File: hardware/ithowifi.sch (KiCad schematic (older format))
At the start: 20 parts, among them J1 Conn_02x03_Odd_Even, J2 conn, Q1 BSS138, Q2 BSS138, U1 WeMos_mini

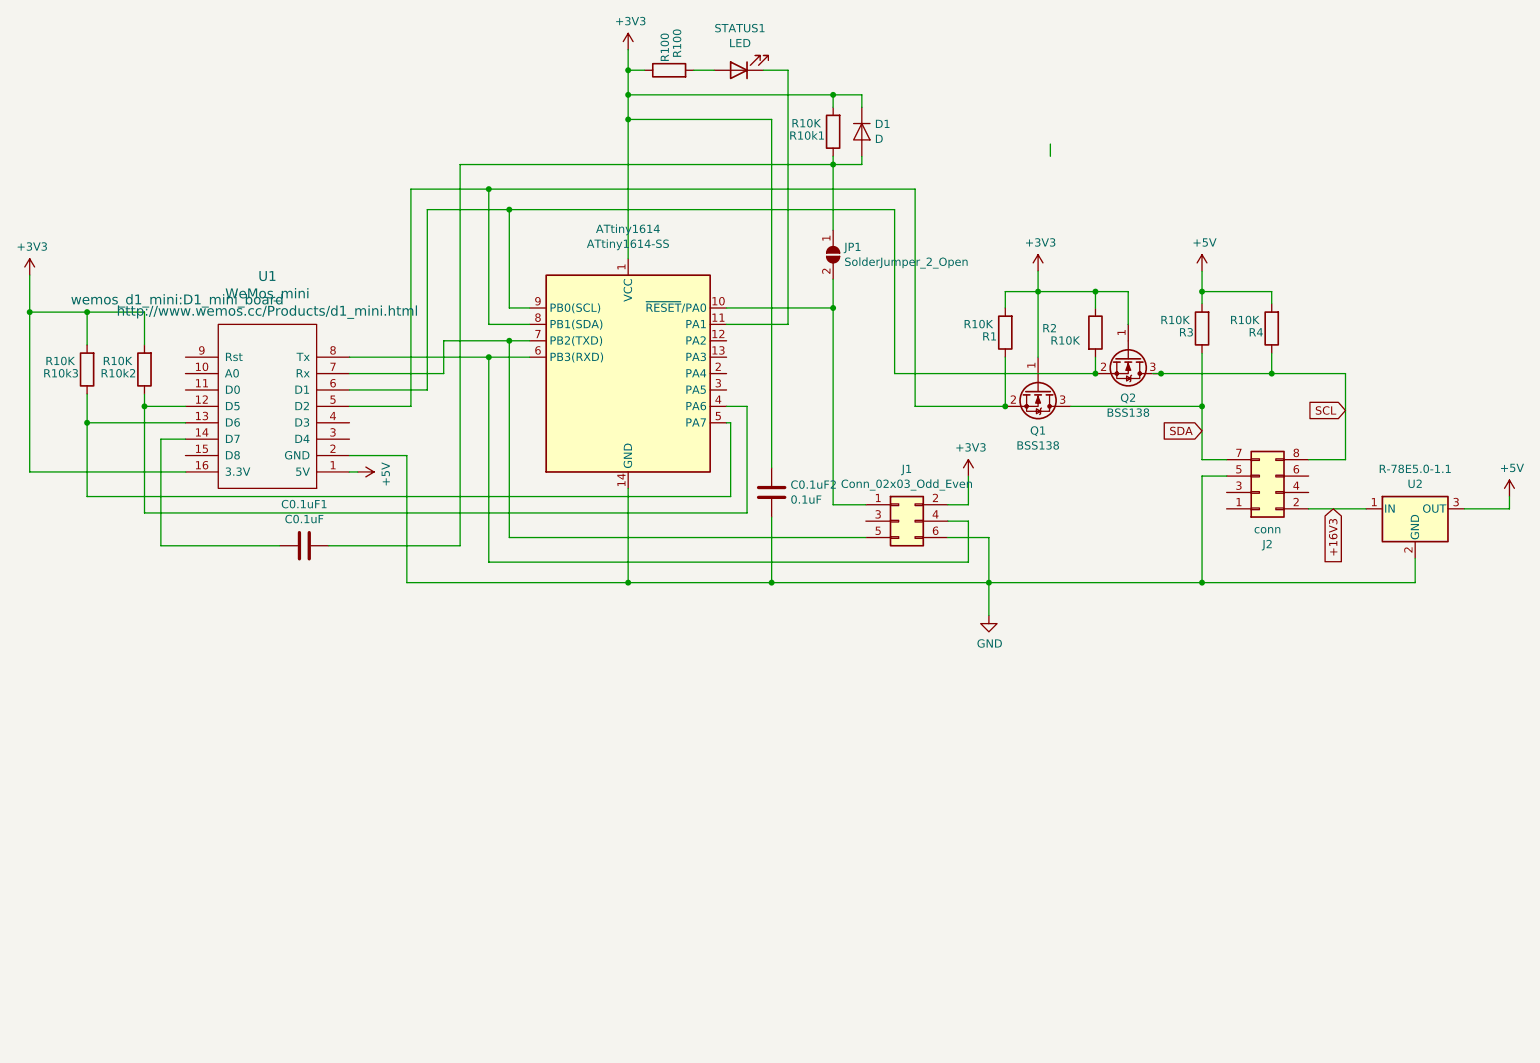
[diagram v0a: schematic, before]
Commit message: Test v2.0
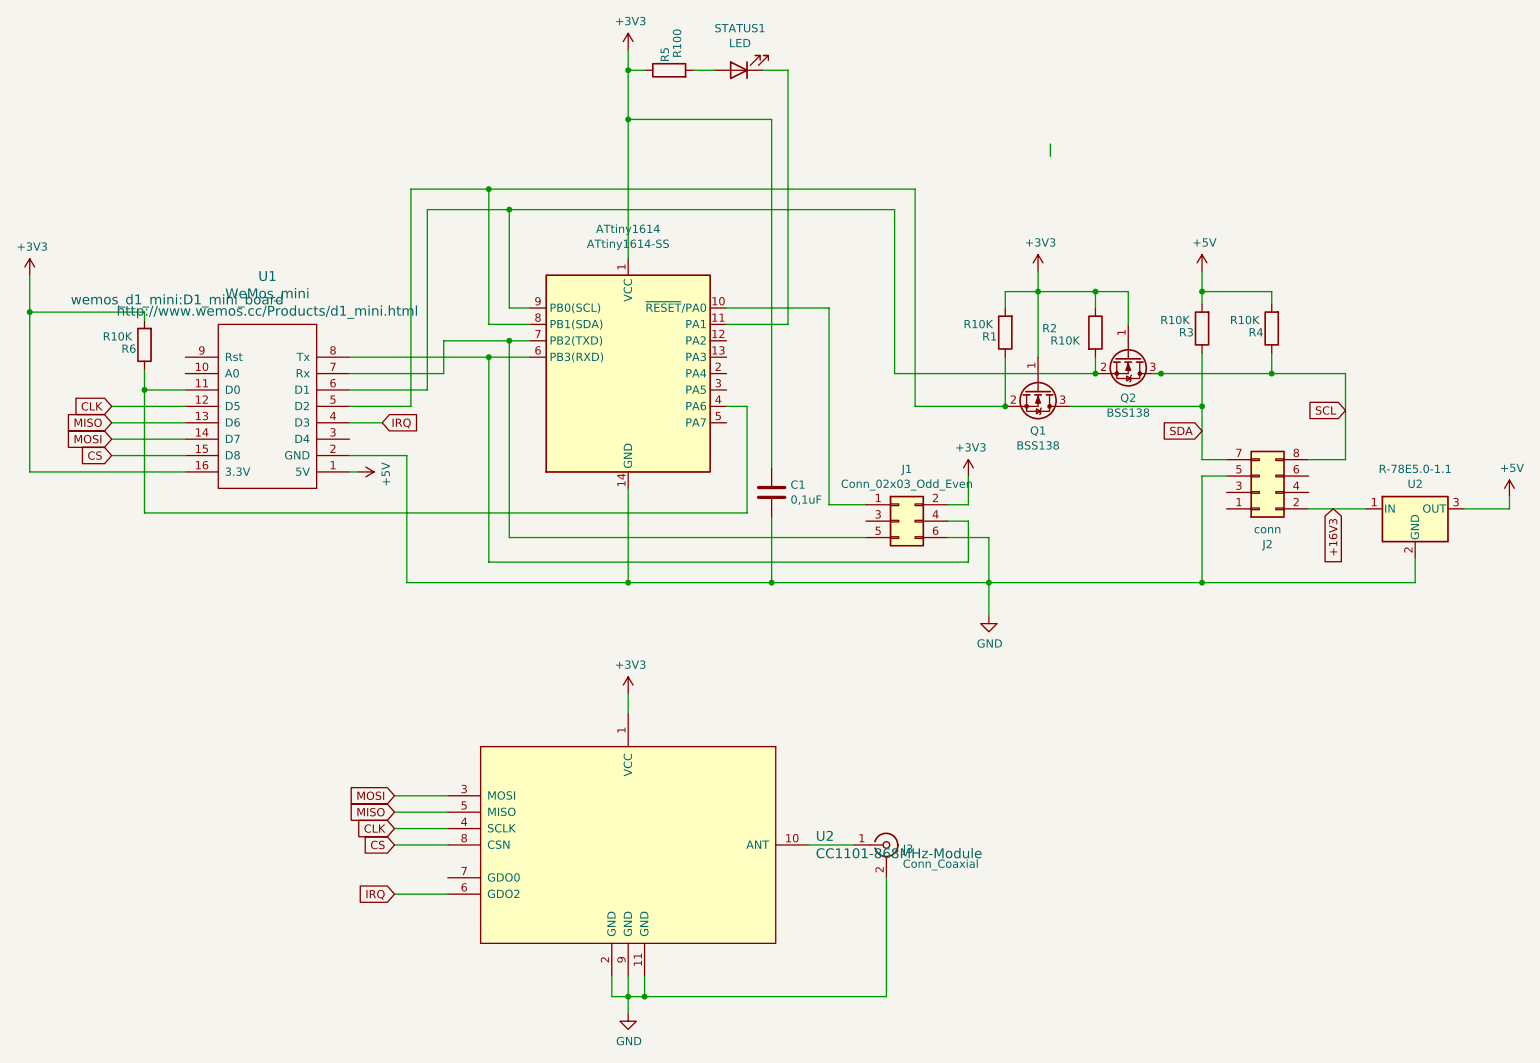
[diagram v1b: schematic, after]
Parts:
- removed C0.1uF1: C0.1uF, Inductor_SMD:L_1206_3216Metric, symbol Device:C
- removed D1: D, Diode_SMD:D_SOD-123, symbol Device:D
- removed JP1: SolderJumper_2_Open, Jumper:SolderJumper-2_P1.3mm_Open_RoundedPad1.0x1.5mm, symbol Jumper:SolderJumper_2_Open
- removed R10k1, R10k3: R10K, Resistor_SMD:R_1206_3216Metric, symbol Device:R
- added J3: Conn_Coaxial, Connector_Coaxial:SMA_Amphenol_132289_EdgeMount, symbol Connector:Conn_Coaxial
- added U2: CC1101-868MHz-Module, nrg_watch:CC1101-868MHz-Module, symbol nrg_watch:CC1101-868MHz-Module
- C1: renamed from C0.1uF2; value 0.1uF -> 0,1uF; footprint Inductor_SMD:L_1206_3216Metric -> Inductor_SMD:L_0805_2012Metric
- Q1, Q2: footprint Package_TO_SOT_SMD:SOT-23W -> Package_TO_SOT_SMD:SOT-23
- R1, R2, R3, R4: footprint Resistor_SMD:R_1206_3216Metric -> Resistor_SMD:R_0805_2012Metric
- R5: renamed from R100; footprint Resistor_SMD:R_1206_3216Metric -> Resistor_SMD:R_0805_2012Metric
- R6: renamed from R10k2; footprint Resistor_SMD:R_1206_3216Metric -> Resistor_SMD:R_0805_2012Metric
- STATUS1: footprint LED_SMD:LED_1206_3216Metric -> LED_SMD:LED_0805_2012Metric
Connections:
- net labels added: CLK, CS, IRQ, MISO, MOSI
- wire segments 122 -> 118
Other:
- moved on the sheet: R6

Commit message: Revert "Test v2.0"
This reverts commit 51a6d60645f7c24e24572af265a76d84da59fee7.
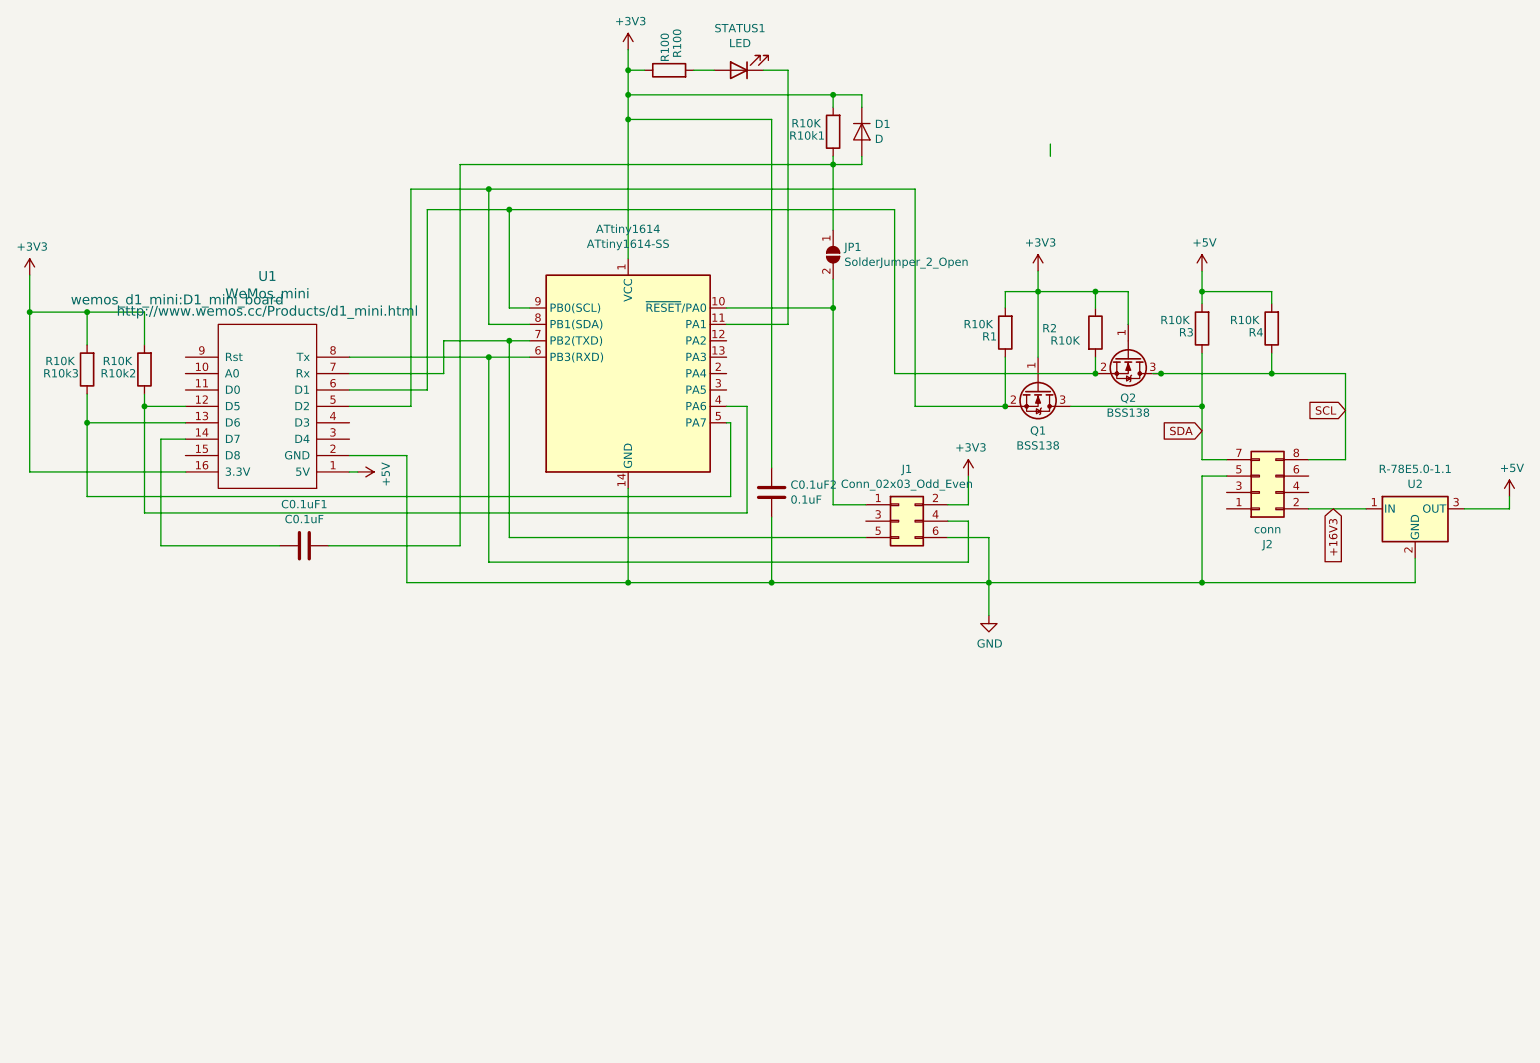
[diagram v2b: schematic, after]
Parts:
- removed J3: Conn_Coaxial, Connector_Coaxial:SMA_Amphenol_132289_EdgeMount, symbol Connector:Conn_Coaxial
- removed U2: CC1101-868MHz-Module, nrg_watch:CC1101-868MHz-Module, symbol nrg_watch:CC1101-868MHz-Module
- added C0.1uF1: C0.1uF, Inductor_SMD:L_1206_3216Metric, symbol Device:C
- added D1: D, Diode_SMD:D_SOD-123, symbol Device:D
- added JP1: SolderJumper_2_Open, Jumper:SolderJumper-2_P1.3mm_Open_RoundedPad1.0x1.5mm, symbol Jumper:SolderJumper_2_Open
- added R10k1, R10k3: R10K, Resistor_SMD:R_1206_3216Metric, symbol Device:R
- C0.1uF2: renamed from C1; value 0,1uF -> 0.1uF; footprint Inductor_SMD:L_0805_2012Metric -> Inductor_SMD:L_1206_3216Metric
- Q1, Q2: footprint Package_TO_SOT_SMD:SOT-23 -> Package_TO_SOT_SMD:SOT-23W
- R1, R2, R3, R4: footprint Resistor_SMD:R_0805_2012Metric -> Resistor_SMD:R_1206_3216Metric
- R100: renamed from R5; footprint Resistor_SMD:R_0805_2012Metric -> Resistor_SMD:R_1206_3216Metric
- R10k2: renamed from R6; footprint Resistor_SMD:R_0805_2012Metric -> Resistor_SMD:R_1206_3216Metric
- STATUS1: footprint LED_SMD:LED_0805_2012Metric -> LED_SMD:LED_1206_3216Metric
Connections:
- net labels removed: CLK, CS, IRQ, MISO, MOSI
- wire segments 118 -> 122
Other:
- moved on the sheet: R10k2
